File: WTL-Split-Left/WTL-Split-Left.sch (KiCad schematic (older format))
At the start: 48 parts, among them J1 MJ-4PP-9, U1 ProMicro

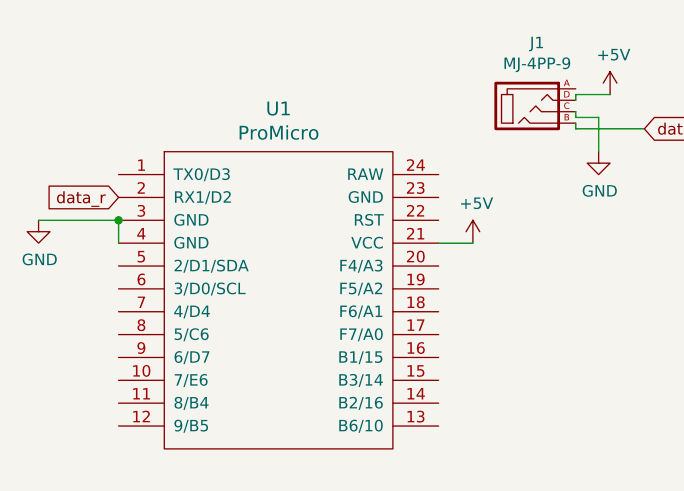
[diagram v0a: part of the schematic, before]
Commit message: this project gonna end up in a bin but ok
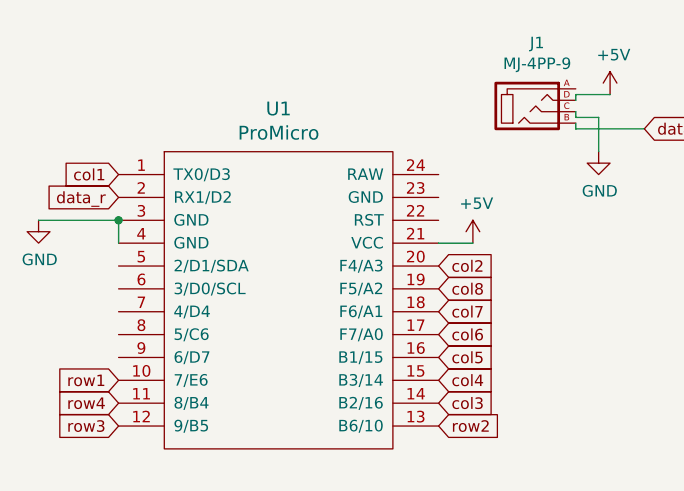
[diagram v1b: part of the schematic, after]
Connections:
- net col1: now also U1.1 (TX0/D3)
- net col2: now also U1.20 (F4/A3)
- net col3: now also U1.14 (B2/16)
- net col4: now also U1.15 (B3/14)
- net col5: now also U1.16 (B1/15)
- net col6: now also U1.17 (F7/A0)
- net col7: now also U1.18 (F6/A1)
- net col8: now also U1.19 (F5/A2)
- net row1: now also U1.10 (7/E6)
- net row2: now also U1.13 (B6/10)
- net row3: now also U1.12 (9/B5)
- net row4: now also U1.11 (8/B4)
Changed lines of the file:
@@
 Connection ~ 1200 4850
 $Comp
-L power:+5V #PWR?
+L power:+5V #PWR0104
 U 1 1 61380FCA
 P 2750 4950
-F 0 "#PWR?" H 2750 4800 50  0001 C CNN
+F 0 "#PWR0104" H 2750 4800 50  0001 C CNN
 F 1 "+5V" H 2765 5123 50  0000 C CNN
 F 2 "" H 2750 4950 50  0001 C CNN
@@
 Wire Wire Line
 	2600 4950 2750 4950
+Text GLabel 1200 4650 0    50   Input ~ 0
+col1
+Text GLabel 2600 5050 2    50   Input ~ 0
+col2
+Text GLabel 2600 5650 2    50   Input ~ 0
+col3
+Text GLabel 2600 5150 2    50   Input ~ 0
+col8
+Text GLabel 2600 5250 2    50   Input ~ 0
+col7
+Text GLabel 2600 5350 2    50   Input ~ 0
+col6
+Text GLabel 2600 5450 2    50   Input ~ 0
+col5
+Text GLabel 2600 5550 2    50   Input ~ 0
+col4
+Text GLabel 2600 5750 2    50   Input ~ 0
+row2
+Text GLabel 1200 5750 0    50   Input ~ 0
+row3
+Text GLabel 1200 5650 0    50   Input ~ 0
+row4
+Text GLabel 1200 5550 0    50   Input ~ 0
+row1
 $EndSCHEMATC

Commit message: I don't remember what i've done
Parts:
- J1: symbol kbd:MJ-4PP-9 -> WTL-Split-Left-rescue:MJ-4PP-9-kbd
- MX14, MX22: footprint MX_Only:MXOnly-2U-NoLED -> MX_Only:MXOnly-2U-ReversedStabilizers-NoLED
- U1: symbol kbd:ProMicro -> WTL-Split-Left-rescue:ProMicro-kbd
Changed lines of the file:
@@
 F 0 "MX14" H 5183 5173 60  0000 C CNN
 F 1 "MX-NoLED" H 5183 5099 20  0000 C CNN
-F 2 "MX_Only:MXOnly-2U-NoLED" H 4525 4925 60  0001 C CNN
+F 2 "MX_Only:MXOnly-2U-ReversedStabilizers-NoLED" H 4525 4925 60  0001 C CNN
 F 3 "" H 4525 4925 60  0001 C CNN
 	1    5150 4950
@@
 F 0 "MX22" H 6983 5773 60  0000 C CNN
 F 1 "MX-NoLED" H 6983 5699 20  0000 C CNN
-F 2 "MX_Only:MXOnly-2U-NoLED" H 6325 5525 60  0001 C CNN
+F 2 "MX_Only:MXOnly-2U-ReversedStabilizers-NoLED" H 6325 5525 60  0001 C CNN
 F 3 "" H 6325 5525 60  0001 C CNN
 	1    6950 5550
@@
 Connection ~ 8000 4900
 $Comp
-L kbd:ProMicro U1
+L WTL-Split-Left-rescue:ProMicro-kbd U1
 U 1 1 614197CC
 P 1900 5200
@@
 data_r
 $Comp
-L kbd:MJ-4PP-9 J1
+L WTL-Split-Left-rescue:MJ-4PP-9-kbd J1
 U 1 1 6141D0A5
 P 3000 4350
